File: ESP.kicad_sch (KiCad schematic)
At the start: 18 parts, among them J7 Conn, U3 ESP32-C3-MINI-1-N4, U5 TCAN1042VDRBRQ1

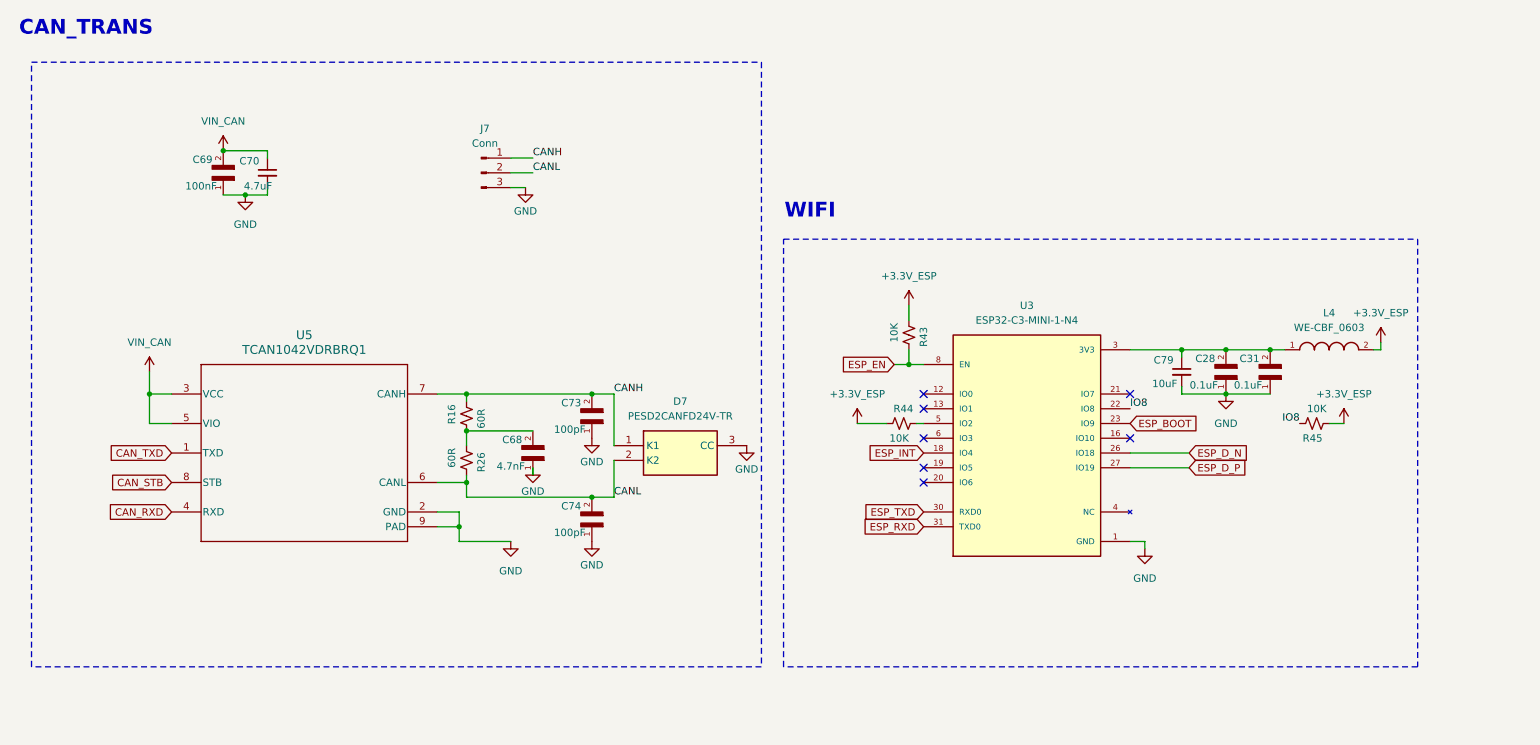
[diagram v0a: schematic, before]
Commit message: new
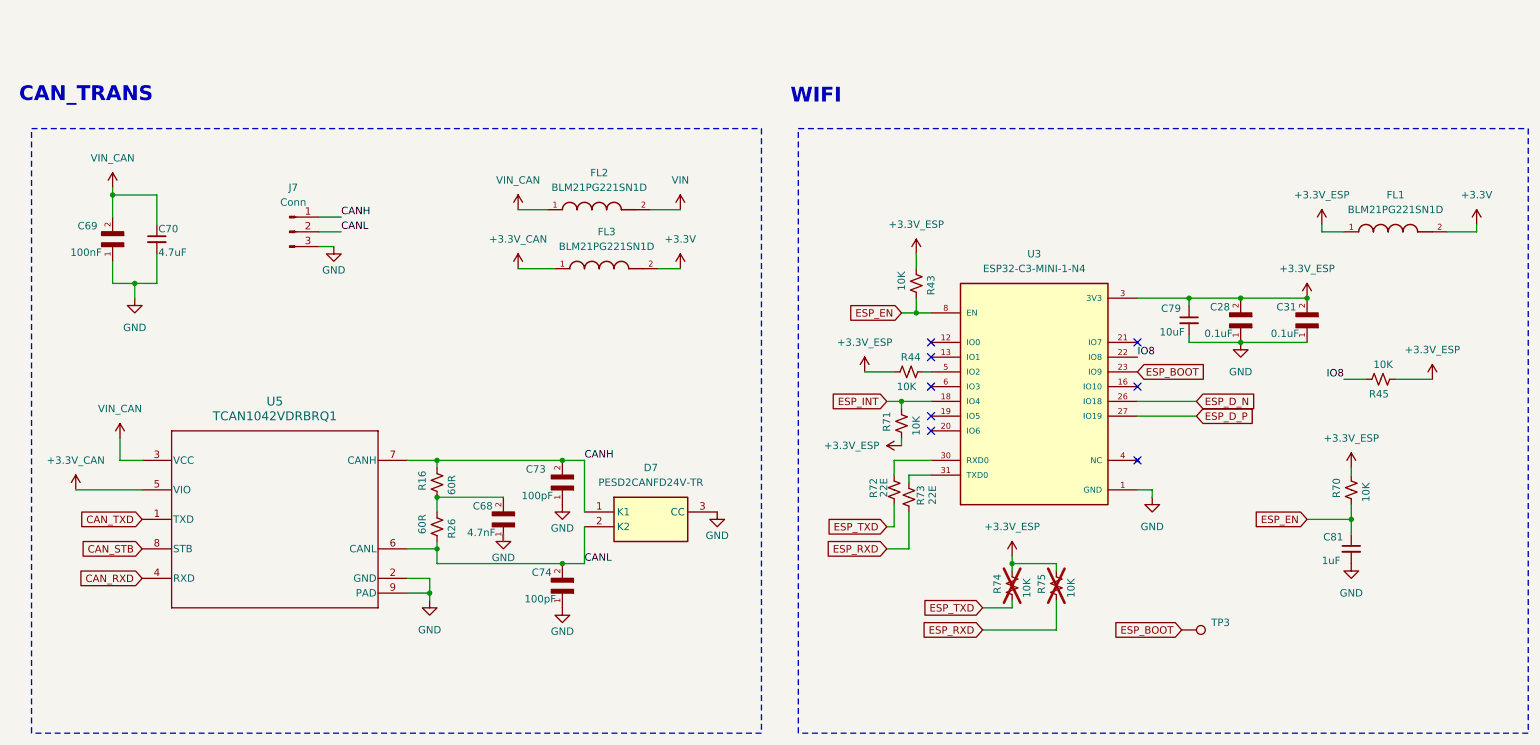
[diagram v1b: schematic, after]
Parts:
- removed L4: WE-CBF_0603, GNSS_Library:WE-CBF_0603_W2.6, symbol WE-CBF_0603:WE-CBF_0603
- added C81: 1uF, Capacitor_SMD:C_0805_2012Metric, symbol Device:C_Small
- added FL1, FL2, FL3: BLM21PG221SN1D, BLM21PG221SN1D:BEADC2012X105N, symbol BLM21PG221SN1D:BLM21PG221SN1D
- added R70, R71, R74, R75: 10K, Resistor_SMD:R_0805_2012Metric, symbol Device:R_Small_US
- added R72, R73: 22E, Resistor_SMD:R_0805_2012Metric, symbol Device:R_Small_US
- added TP3: TestPoint, TestPoint:TestPoint_Pad_D2.0mm, symbol Connector:TestPoint
- U3: footprint Module:XCVR_ESP32-C3-MINI-1-N4 -> GNSS:XCVR_ESP32-C3-MINI-1-N4
- U5: footprint GNSS_Library:DRB0008F -> GNSS:DRB0008F
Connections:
- net +3.3V_ESP: now also C28.2, C31.2, C79.1, U3.3 (3V3), FL1.1, R70.2, R71.1, R74.2, R75.2
- net ESP_BOOT: now also TP3.1
- net ESP_EN: now also C81.1, R70.1
- net ESP_INT: now also R71.2
- net ESP_RXD: now also R73.1, R75.1; no longer U3.31 (TXD0)
- net ESP_TXD: now also R72.1, R74.1; no longer U3.30 (RXD0)
- net GND: now also C81.2
- net VIN_CAN: now also FL2.1; no longer U5.5 (VIO)
- new net: R73.2, U3.31 (TXD0)
- new net: R72.2, U3.30 (RXD0)
- new net +3.3V: FL1.2, FL3.2
- new net +3.3V_CAN: FL3.1, U5.5 (VIO)
- new net VIN: FL2.2
- no-connect marks 7 -> 8
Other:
- moved on the sheet: C28, C31, C68, C69, C70, C73, C74, C79, D7, J7, R16, R26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
